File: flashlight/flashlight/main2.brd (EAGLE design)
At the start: 20 x 20 mm, 10 parts

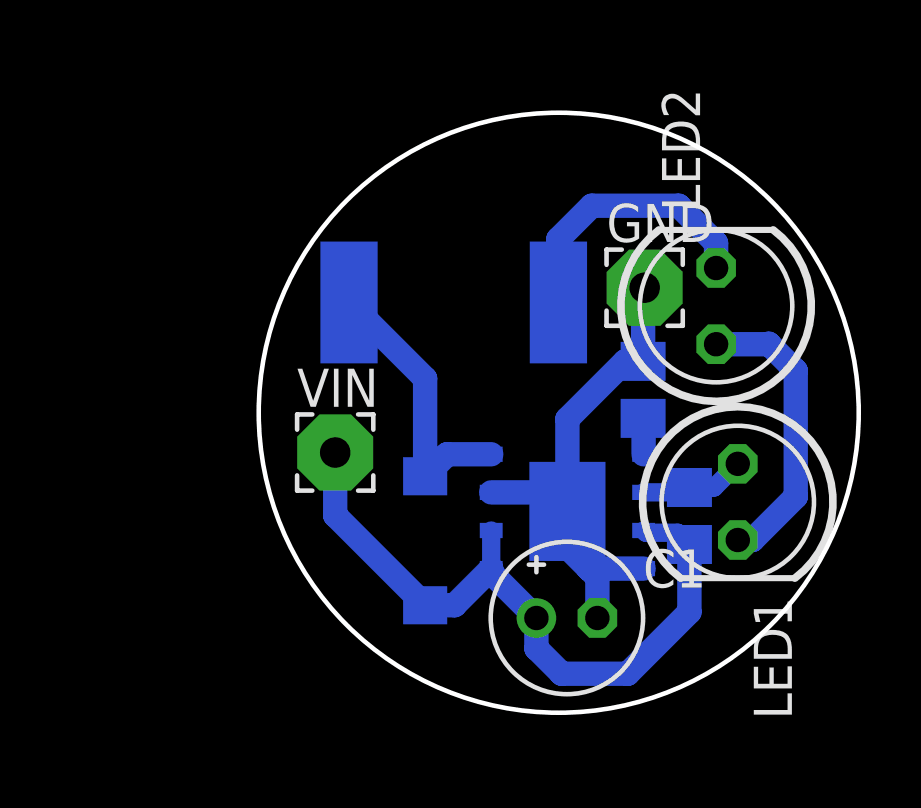
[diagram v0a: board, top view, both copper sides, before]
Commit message: updated project
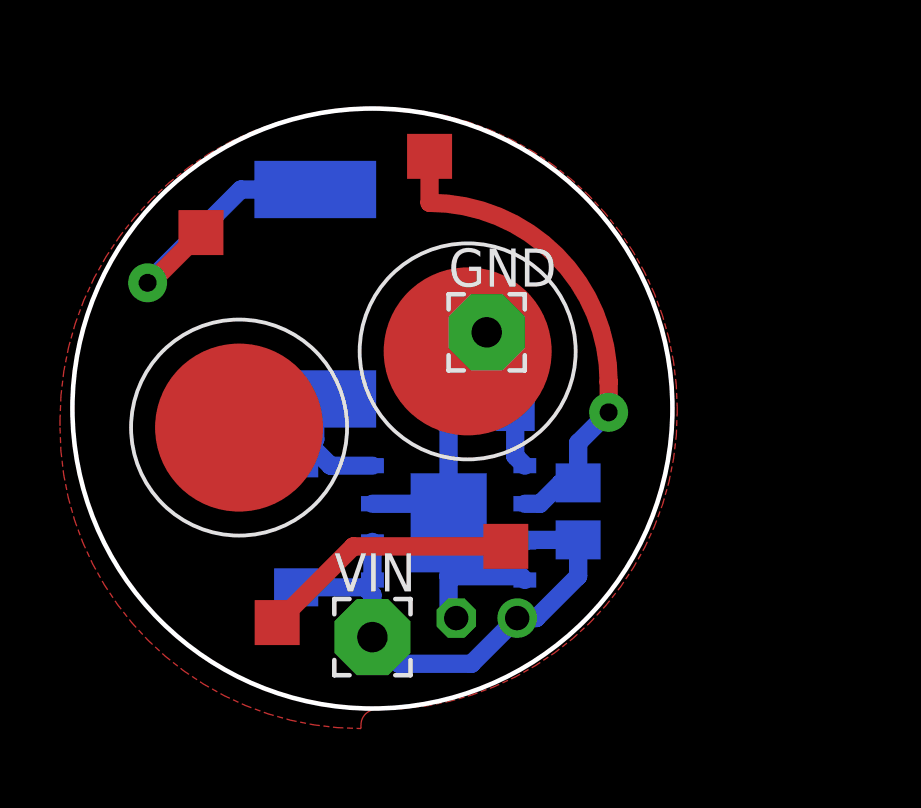
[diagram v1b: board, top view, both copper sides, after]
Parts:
- LED1, LED2: value (none) -> COBLED; device led:LED5MM -> 7_segment_lib:COBLED
- moved LED2 16.4 mm to (-8.26, 1.91)
- moved LED1 10.3 mm to (-0.64, 4.45)
- moved VIN 6.28 mm to (-3.81, -5.08)
- moved GND 5.47 mm to (0.00, 5.08)
- moved C2 5.25 mm to (0.00, 2.54), turned to 0 degrees
- moved U$3 4.62 mm to (-5.71, 6.35), turned to 270 degrees
- moved D1 4.34 mm to (-6.35, -1.27)
- moved U$1 3.98 mm to (-1.27, -1.27)
- moved R1 3.71 mm to (3.05, -0.89)
- moved C1 2.67 mm to (0.00, -4.45), flipped to the bottom
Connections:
- new net PLANE: LED1.P$3, LED2.P$3
- net N$1: now also LED1.P$2, LED2.P$1; no longer LED1.K, LED2.A
- net N$5: now also LED1.P$1; no longer LED1.A
- net N$7: now also LED2.P$2; no longer LED2.K
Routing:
- net N$5: track 3.53 -> 15.8 mm, vias 0 -> 1
- net N$3: track 23.9 -> 17.1 mm
- net N$6: track 9.35 -> 4.62 mm
- net N$2: track 17.5 -> 15.6 mm
- net N$1: track 9.76 -> 8.67 mm
- net N$4: track 1.20 -> 2.04 mm
- net N$7: track 9.18 -> 9.35 mm, vias 0 -> 1
- added copper zone on layer 1, net PLANE
